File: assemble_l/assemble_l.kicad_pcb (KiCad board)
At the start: 2 copper layers, 128.5 x 102.6 mm, 51 parts, among them SW1 SW_Push, SW10 SW_Push, SW11 SW_Push, SW12 SW_Push, SW13 SW_Push, SW14 SW_Push, SW15 SW_Push, SW16 SW_Push, SW17 SW_Push, SW18 SW_Push, SW19 SW_Push, SW2 SW_Push, SW20 SW_Push, SW21 SW_Push, SW22 SW_Push, SW23 SW_SPDT, SW3 SW_Push, SW4 SW_Push, SW5 SW_Push, SW6 SW_Push, SW7 SW_Push, SW8 SW_Push, SW9 SW_Push, U1 Micon_BLEMicroPro

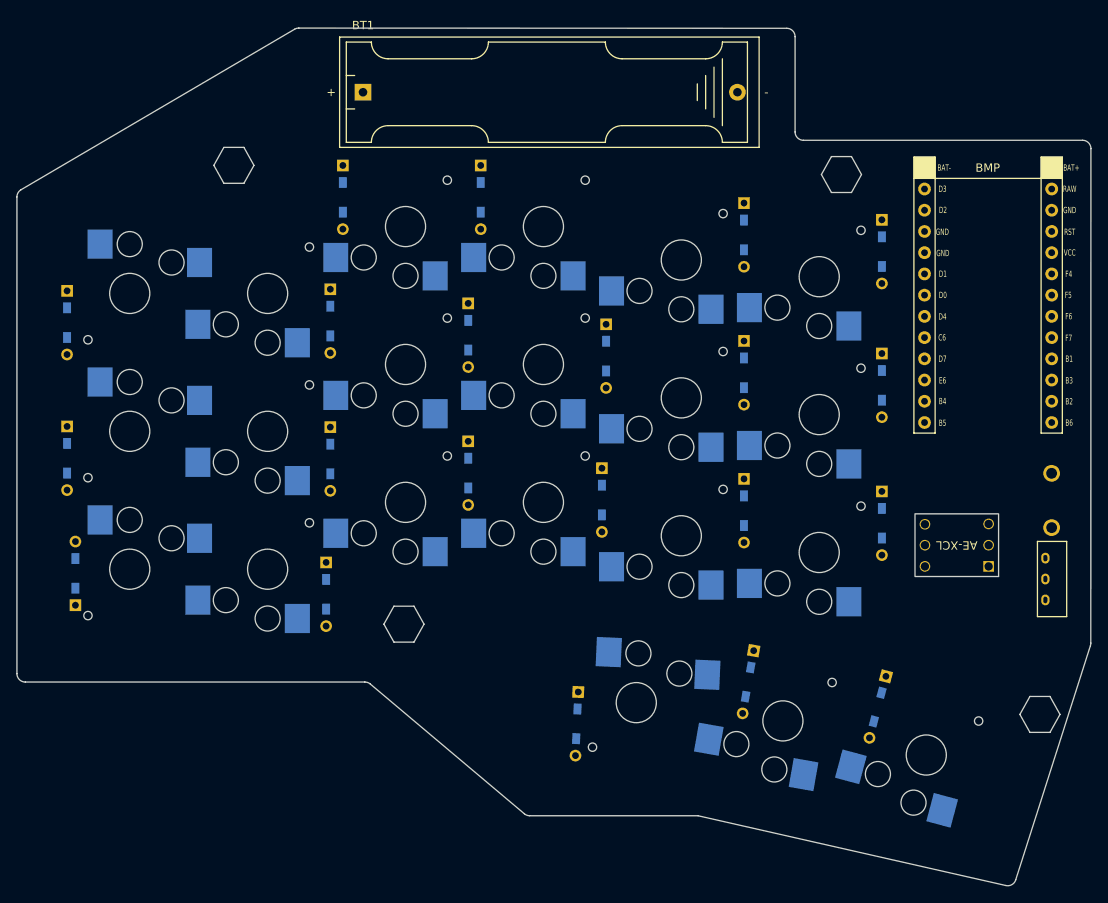
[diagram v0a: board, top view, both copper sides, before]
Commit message: feat: wiring in left
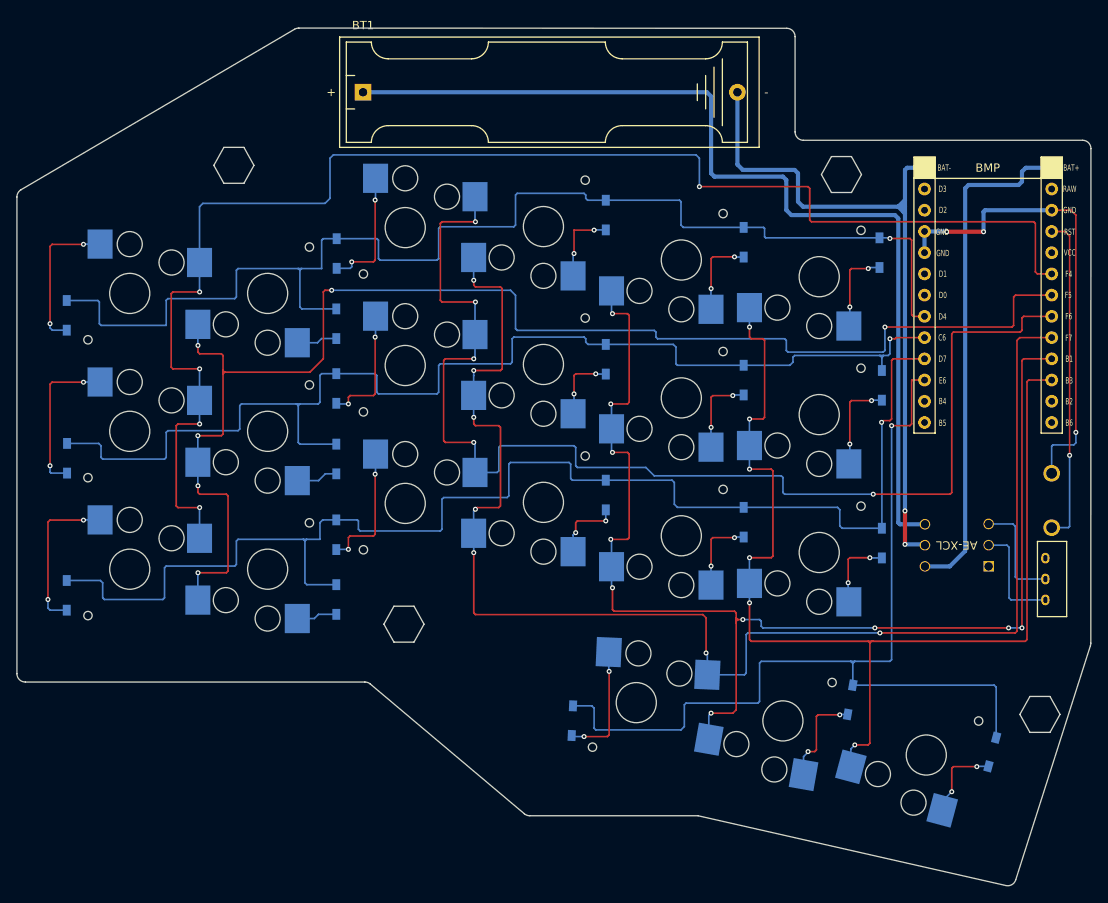
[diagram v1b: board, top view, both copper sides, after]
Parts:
- D1, D10, D11, D12, D13, D14, D15, D16, D17, D18, D19, D2, D20, D21, D3, D4, D5, D6, D7, D8, D9: footprint kbd_Parts:Diode_TH_SMD -> kbd_Parts:Diode_SMD
- moved D6 48.1 mm to (94.8, 110.0)
- moved SW6 44.2 mm to (86.5, 106.4)
- moved D8 18.8 mm to (94.8, 84.8)
- moved D7 18.5 mm to (94.8, 68.6)
- moved SW9 18.2 mm to (103.0, 98.5), turned to 180 degrees
- moved SW7 16.4 mm to (103.0, 65.5), turned to 180 degrees
- moved SW8 16.4 mm to (103.0, 82.0), turned to 180 degrees
- moved D10 15.1 mm to (127.0, 64.0)
- moved D21 14.7 mm to (173.2, 128.2)
- moved D17 12.4 mm to (156.2, 122.0)
- moved D9 7.23 mm to (94.8, 102.2)
- moved D3 2.82 mm to (62.5, 109.5), turned to -90 degrees
- moved D20 2.38 mm to (160.0, 103.2)
- moved D16 1.38 mm to (143.5, 100.8)
- moved D1 0.88 mm to (62.5, 76.0)
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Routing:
- net Col0: track 0.00 -> 172.5 mm, vias 0 -> 5
- net Col3: track 0.00 -> 170.7 mm, vias 0 -> 7
- net Col1: track 0.00 -> 166.9 mm, vias 0 -> 6
- net Row2: track 0.00 -> 158.7 mm, vias 0 -> 1
- net Col4: track 0.00 -> 150.6 mm, vias 0 -> 10
- net Row0: track 0.00 -> 148.4 mm, vias 0 -> 1
- net Col2: track 0.00 -> 145.8 mm, vias 0 -> 5
- net Row1: track 0.00 -> 139.6 mm, vias 0 -> 1
- net Col5: track 0.00 -> 133.1 mm, vias 0 -> 6
- net Net-(BT1-+): track 0.00 -> 117.5 mm
- net Row3: track 0.00 -> 112.3 mm, vias 0 -> 1
- net Bat-: track 0.00 -> 84.9 mm, vias 0 -> 2
- net Bat+: track 0.00 -> 61.3 mm
- net GND: track 0.00 -> 56.9 mm, vias 0 -> 3
- net Reset: track 0.00 -> 39.3 mm, vias 0 -> 1
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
